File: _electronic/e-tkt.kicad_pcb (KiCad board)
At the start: 4 copper layers, 99.6 x 76.2 mm, 111 parts, among them J1 Conn_01x03_Pin, J2 Conn_01x03_Pin, J3 Conn_01x03_Pin, SW1 SW_SPDT, U1 HUSB237-AA001-DN06R

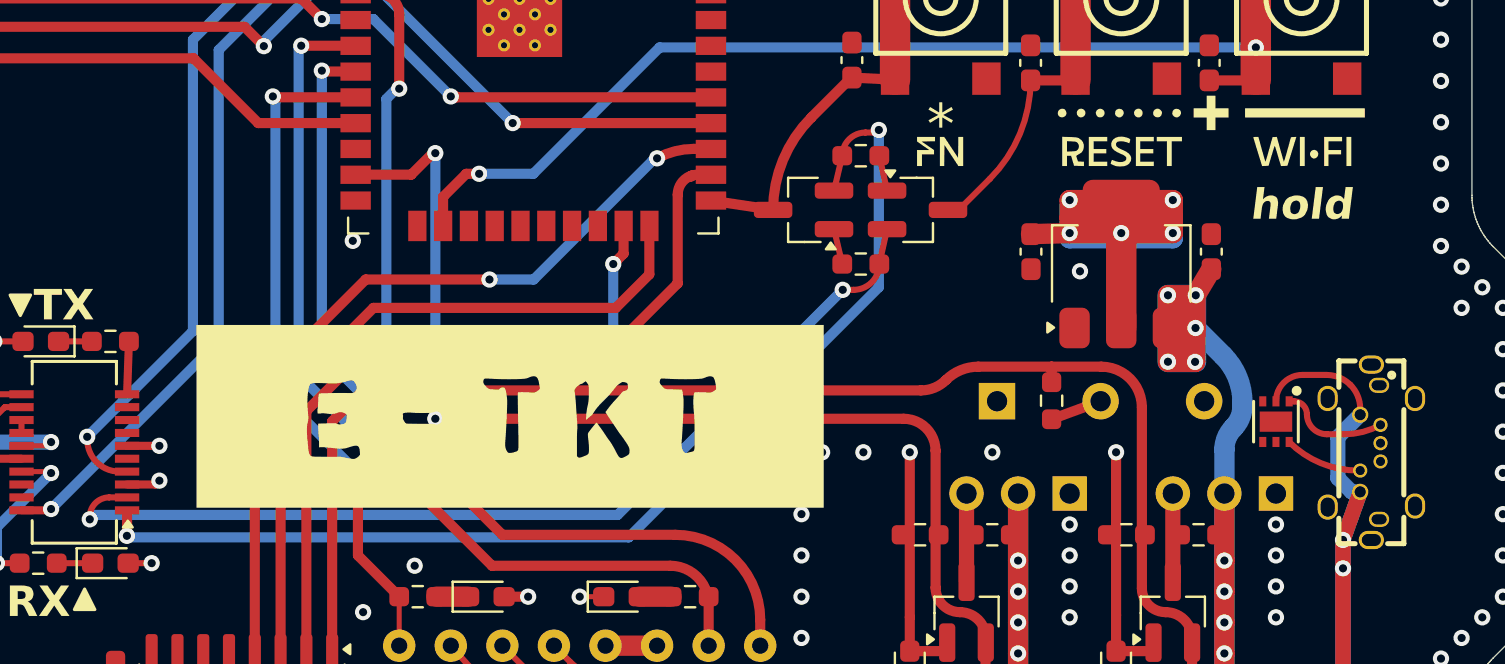
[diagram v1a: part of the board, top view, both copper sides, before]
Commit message: sturdify again
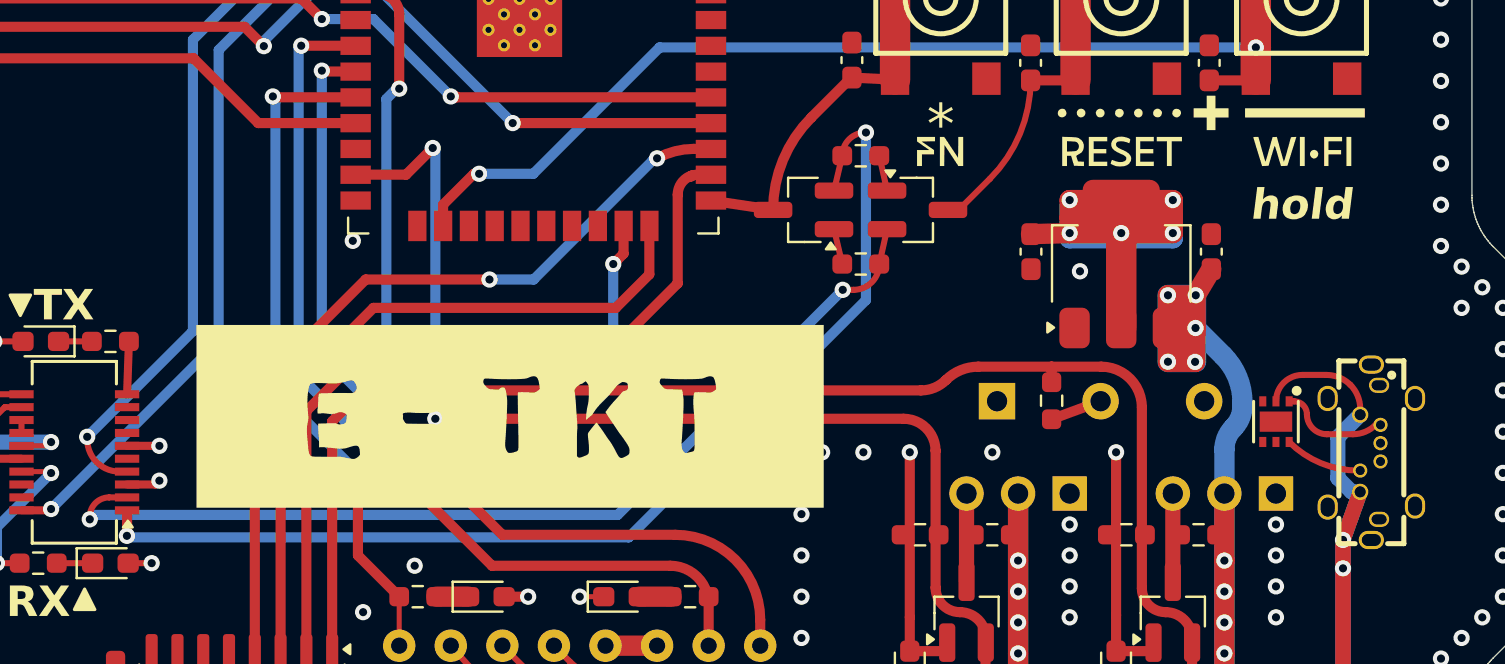
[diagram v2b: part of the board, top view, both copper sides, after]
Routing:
- net DTR: track 55.2 -> 54.1 mm
